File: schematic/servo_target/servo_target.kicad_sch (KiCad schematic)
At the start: 14 parts, among them M1 Motor_Servo, M2 Motor_Servo, M3 Motor_Servo, M4 Motor_Servo, U1 74HC595

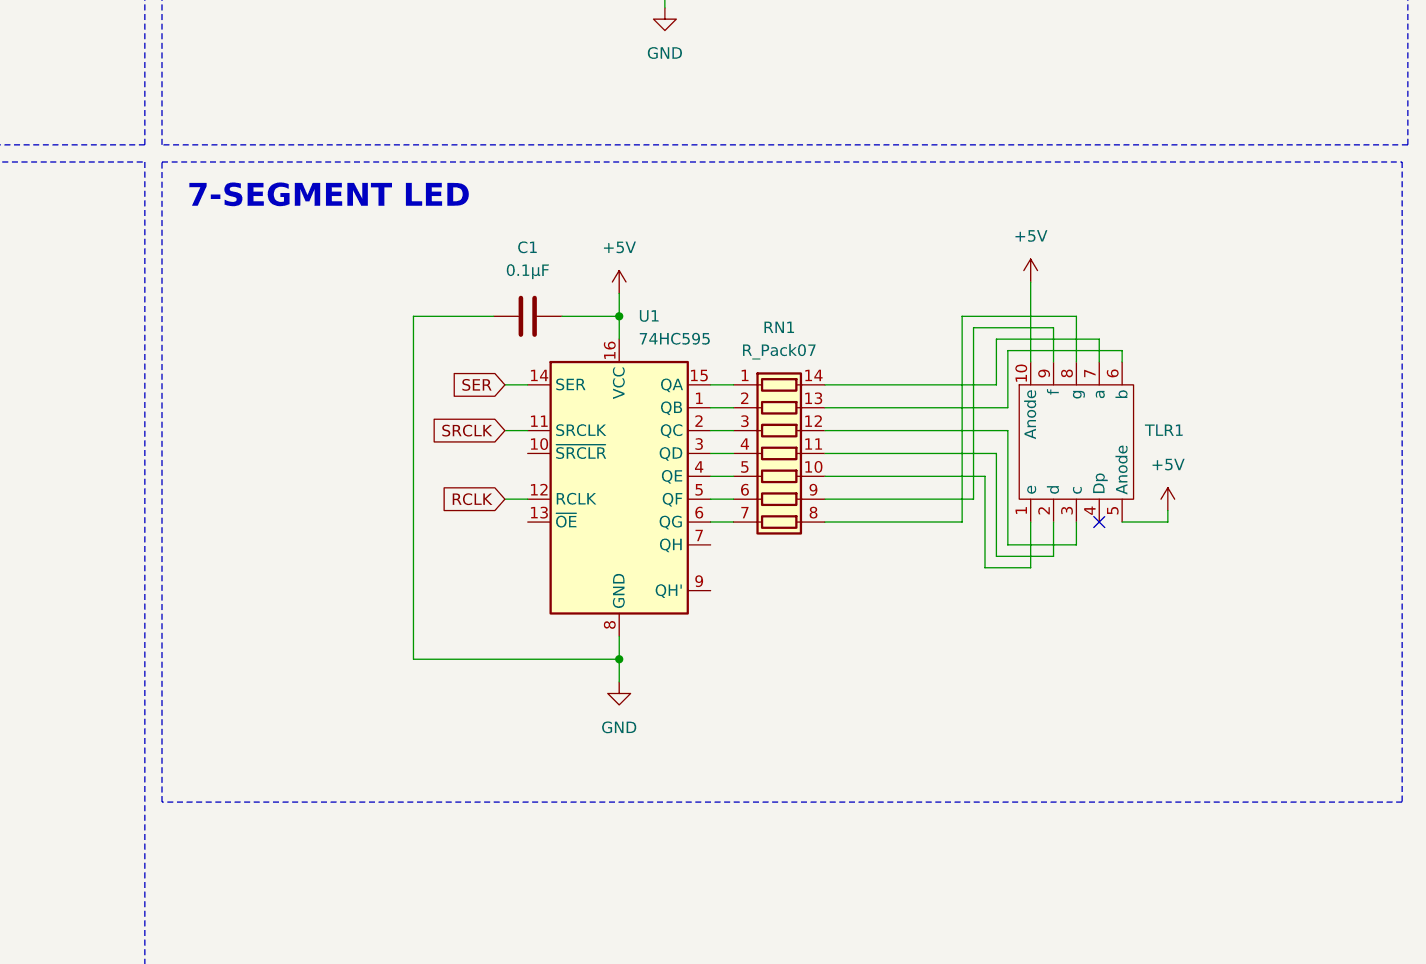
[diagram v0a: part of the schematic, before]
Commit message: 🩹 回路図を修正
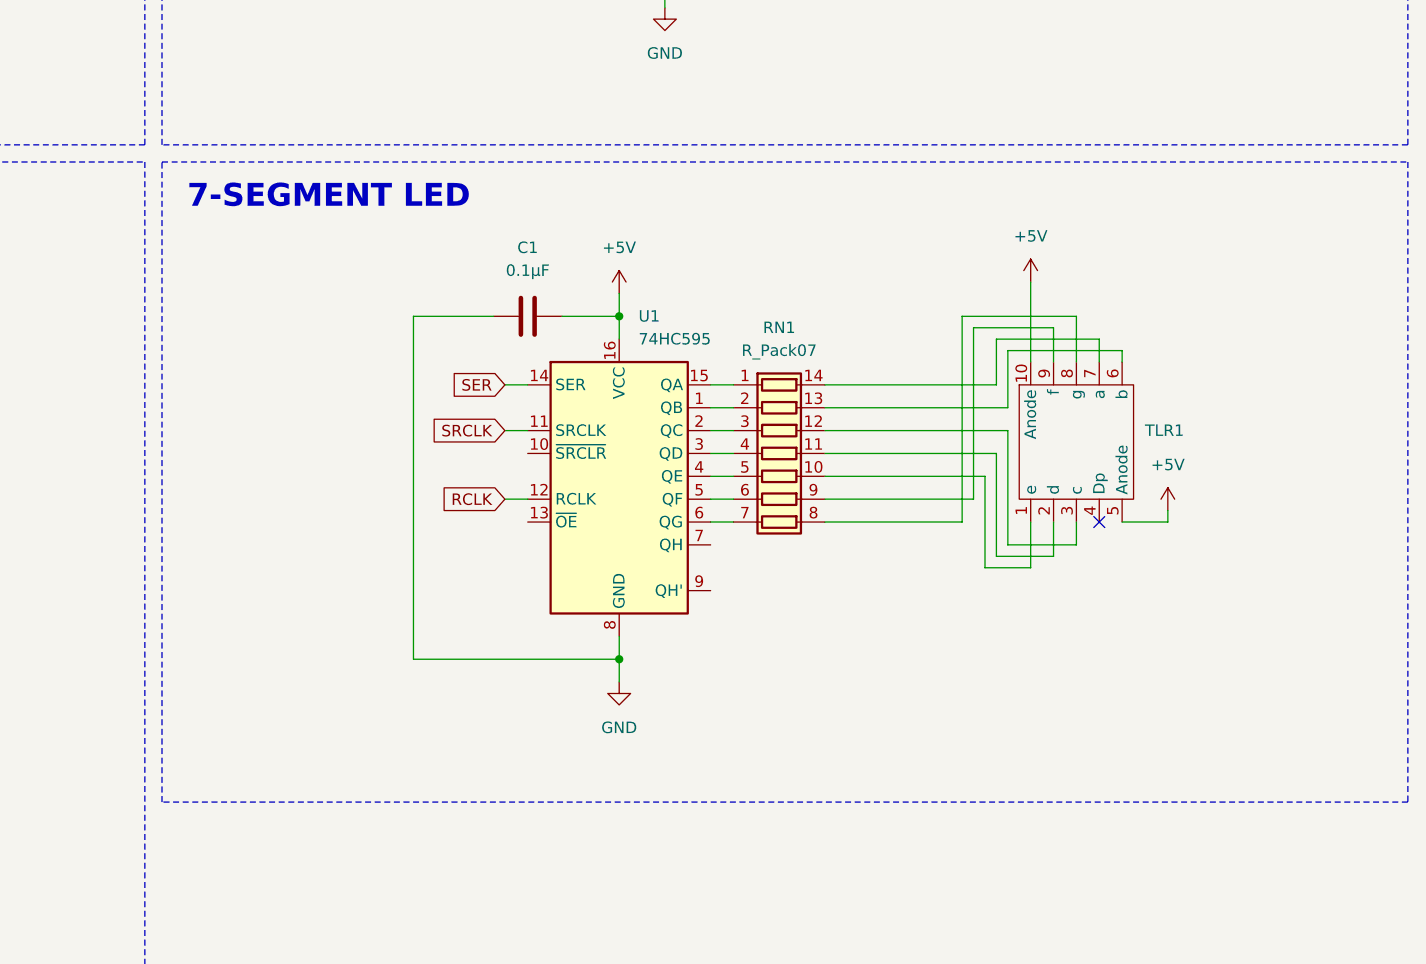
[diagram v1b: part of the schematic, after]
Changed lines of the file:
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@@
 	(rectangle
 		(start 144.78 93.345)
-		(end 282.575 164.465)
+		(end 283.21 164.465)
 		(stroke
 			(width 0)
